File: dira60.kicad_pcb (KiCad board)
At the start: 2 copper layers, 332.4 x 94.5 mm, 203 parts, among them U0 ATmega32U4-AU, X0 XTAL_GND

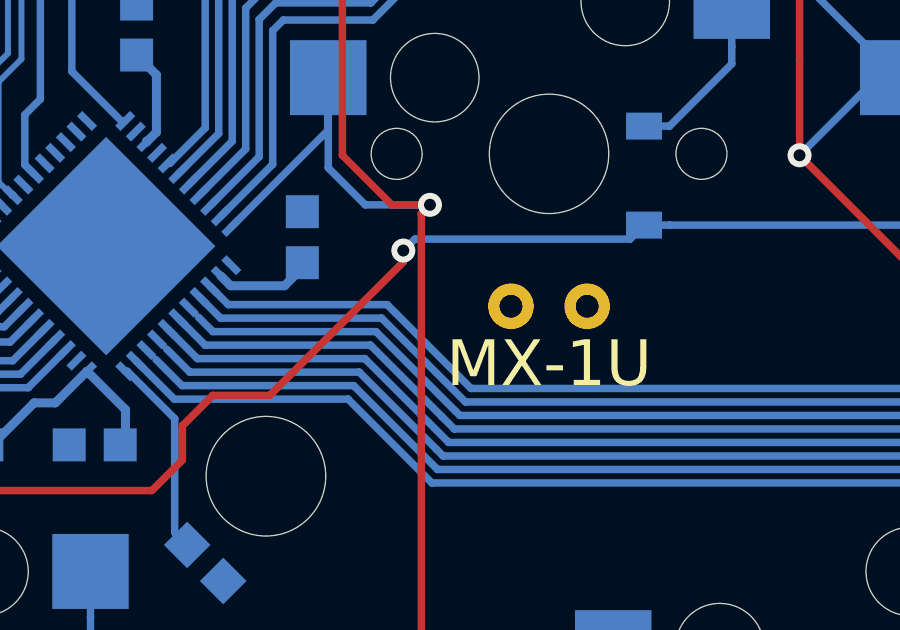
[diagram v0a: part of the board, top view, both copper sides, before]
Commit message: Run drc
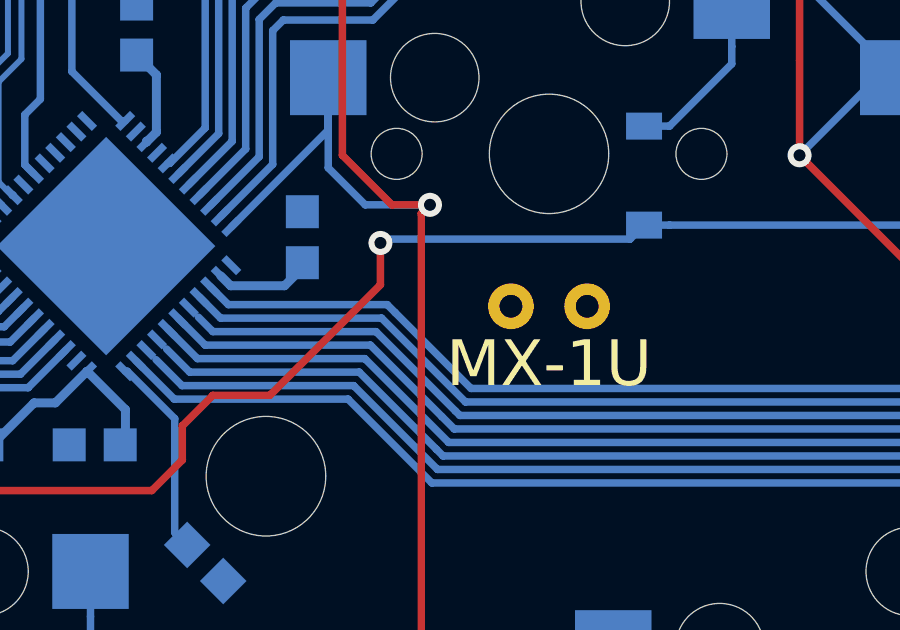
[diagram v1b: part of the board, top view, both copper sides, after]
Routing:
- net ROW2: track 279.2 -> 279.7 mm
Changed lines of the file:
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@@
   (segment (start 282.381783 44.568355) (end 282.381783 43.92002) (width 0.25) (layer B.Cu) (net 36))
   (segment (start 282.381783 43.92002) (end 282.381783 42.42002) (width 0.25) (layer B.Cu) (net 36))
-  (segment (start 50.991384 69.342) (end 43.815 69.342) (width 0.25) (layer B.Cu) (net 37))
-  (segment (start 51.458355 68.875029) (end 50.991384 69.342) (width 0.25) (layer B.Cu) (net 37))
-  (segment (start 43.815 69.342) (end 43.434 69.723) (width 0.25) (layer B.Cu) (net 37))
-  (segment (start 43.434 69.723) (end 43.434 70.104) (width 0.25) (layer F.Cu) (net 37))
-  (segment (start 43.434 70.104) (end 38.989 74.549) (width 0.25) (layer F.Cu) (net 37))
   (segment (start 24.376949 73.024997) (end 17.971497 73.024997) (width 0.25) (layer B.Cu) (net 37))
   (segment (start 17.971497 73.024997) (end 17.0815 72.135) (width 0.25) (layer B.Cu) (net 37))
@@
   (segment (start 16.509 72.135) (end 17.0815 72.135) (width 0.25) (layer B.Cu) (net 37))
   (segment (start 17.0815 72.009) (end 17.0815 72.135) (width 0.25) (layer B.Cu) (net 37))
-  (via (at 43.434 69.723) (size 0.8) (drill 0.4) (layers F.Cu B.Cu) (net 37))
+  (via (at 42.672 69.469) (size 0.8) (drill 0.4) (layers F.Cu B.Cu) (net 37))
   (segment (start 51.458355 68.875029) (end 51.308355 68.875029) (width 0.25) (layer B.Cu) (net 37))
   (segment (start 272.333448 68.941695) (end 241.525101 68.941695) (width 0.25) (layer B.Cu) (net 37))
@@
   (segment (start 51.458355 68.875029) (end 52.308355 68.875029) (width 0.25) (layer B.Cu) (net 37))
   (segment (start 52.308355 68.875029) (end 70.458363 68.875029) (width 0.25) (layer B.Cu) (net 37))
+  (segment (start 42.799 69.342) (end 42.672 69.469) (width 0.25) (layer B.Cu) (net 37))
+  (segment (start 51.458355 68.875029) (end 50.991384 69.342) (width 0.25) (layer B.Cu) (net 37))
+  (segment (start 50.991384 69.342) (end 42.799 69.342) (width 0.25) (layer B.Cu) (net 37))
+  (segment (start 38.989 74.549) (end 42.672 70.866) (width 0.25) (layer F.Cu) (net 37))
+  (segment (start 42.672 70.866) (end 42.672 69.469) (width 0.25) (layer F.Cu) (net 37))
   (segment (start 14.859 67.31) (end 15.5565 67.31) (width 0.25) (layer B.Cu) (net 38))
   (segment (start 15.5565 67.31) (end 17.0815 68.835) (width 0.25) (layer B.Cu) (net 38))
